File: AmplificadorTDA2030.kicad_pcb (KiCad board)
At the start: 2 copper layers, 76 x 60 mm, 45 parts, among them J1 R_Speaker, J2 SJ1-3523N, J3 DC-005, J4 L_Speaker, U1 TDA2030, U2 TDA2030

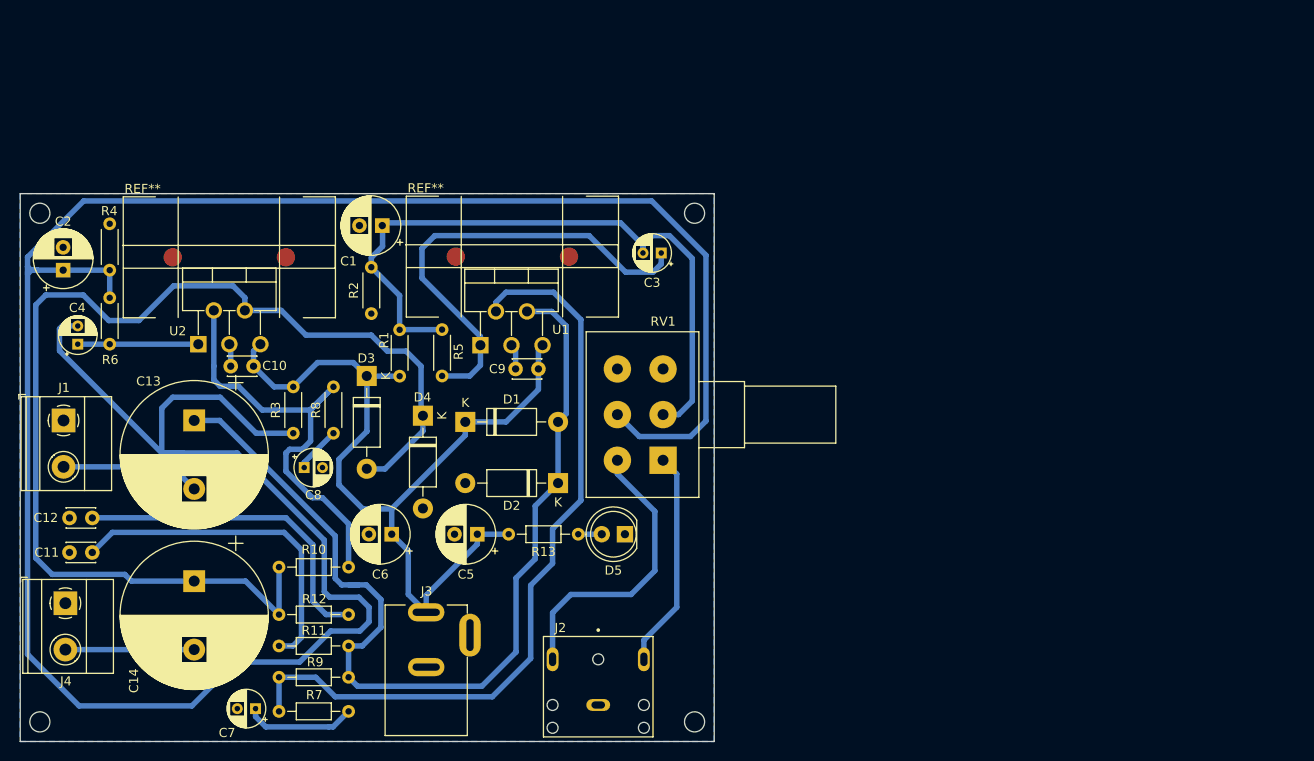
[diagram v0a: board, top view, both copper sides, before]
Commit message: Ruteo
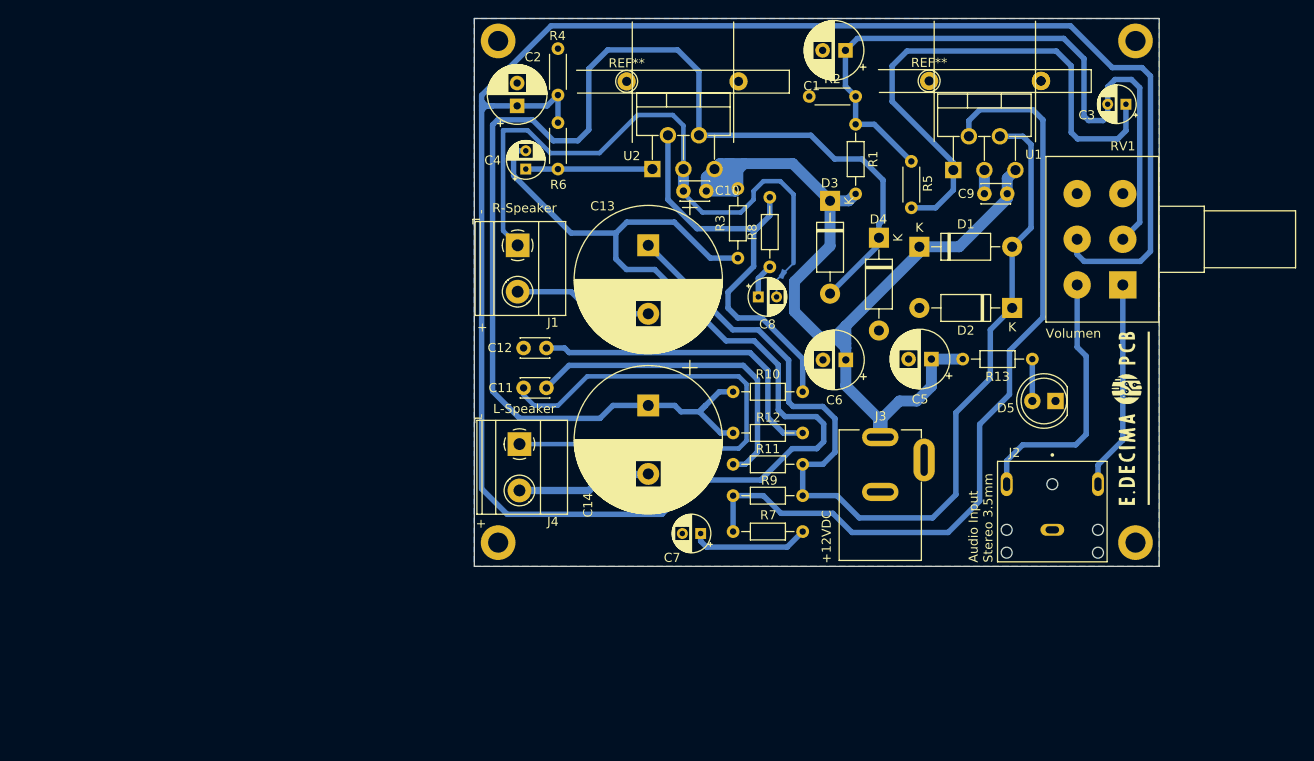
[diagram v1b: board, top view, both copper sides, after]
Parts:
- removed the ? at (136.6, 84.8)
- removed the ? at (64.8, 84.8)
- removed the ? at (64.8, 140.4)
- removed the ? at (136.6, 140.4)
- removed the REF** at (116.6, 89.5)
- removed the REF** at (85.6, 89.6)
- added ? (x2): , , F.Cu at (174.5, 70.3)
- added ?: , , F.Cu at (115.0, 120.8)
- added ?: , , F.Cu at (141.4, 70.3)
- added G***: LOGO, Logo_Image:Logo1_Decima 30mm, F.Cu at (184.2, 107.2)
- added REF**: TestPoint_THTPad_D2.0mm_Drill1.0mm, TestPoint:TestPoint_THTPad_D2.0mm_Drill1.0mm, F.Cu at (129.1, 70.3)
- added REF**: TestPoint_THTPad_D2.0mm_Drill1.0mm, TestPoint:TestPoint_THTPad_D2.0mm_Drill1.0mm, F.Cu at (162.2, 70.3)
- added REF**: MountingHole_2.2mm_M2_DIN965_Pad, MountingHole:MountingHole_2.2mm_M2_DIN965_Pad, F.Cu at (184.8, 120.8)
- added REF**: MountingHole_2.2mm_M2_DIN965_Pad, MountingHole:MountingHole_2.2mm_M2_DIN965_Pad, F.Cu at (115.0, 65.9)
- added REF**: MountingHole_2.2mm_M2_DIN965_Pad, MountingHole:MountingHole_2.2mm_M2_DIN965_Pad, F.Cu at (184.8, 65.9)
- R1, R3, R8: footprint Resistor_THT:R_Axial_DIN0204_L3.6mm_D1.6mm_P5.08mm_Horizontal -> Resistor_THT:R_Axial_DIN0204_L3.6mm_D1.6mm_P7.62mm_Horizontal
- moved U1 55.2 mm to (164.9, 80.0)
- moved C9 54.8 mm to (168.3, 82.6)
- moved R1 54.8 mm to (154.2, 75.0)
- moved R5 54.6 mm to (160.3, 79.1)
- moved D3 54.2 mm to (151.4, 83.4)
- moved C1 54.2 mm to (153.1, 66.9)
- moved RV1 53.9 mm to (183.4, 92.6)
- moved D4 53.6 mm to (156.7, 87.4)
- moved R11 53.6 mm to (140.8, 112.2)
- moved R12 53.6 mm to (148.4, 108.8)
- moved R9 53.6 mm to (148.4, 115.7)
- moved R2 53.5 mm to (149.1, 72.0), turned to 0 degrees
- moved R7 53.5 mm to (148.4, 119.6)
- moved C3 53.4 mm to (183.8, 72.8)
- moved C14 53.3 mm to (131.5, 105.8)
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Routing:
- net GND: track 5.46 -> 132.7 mm
- net Net-(D3-A): track 126.8 -> 142.6 mm
- net /V+: track 96.6 -> 107.2 mm
- net /L_Input: track 288.1 -> 277.8 mm
- net Net-(U1-+): track 50.1 -> 59.6 mm
- net Net-(U1--): track 85.3 -> 89.2 mm
- net /R_Input: track 75.1 -> 78.0 mm
- net Net-(J2-Pad3): track 32.0 -> 29.2 mm
- net Net-(U2--): track 49.3 -> 47.2 mm
- net Net-(D5-A): track 2.58 -> 4.59 mm
- net Net-(C8-Pad1): track 5.09 -> 3.81 mm
- net Net-(C12-Pad2): track 36.1 -> 34.9 mm
- net Net-(C11-Pad2): track 37.0 -> 35.9 mm
- net Net-(J2-Pad2): track 23.9 -> 22.9 mm
- net Net-(C7-Pad1): track 12.2 -> 13.0 mm
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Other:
- board size 76 x 60 mm -> 75 x 60 mm
- board text added: "+"
- board text added: "+12VDC"
- board text added: "-"
- board text added: "Audio Input Stereo 3.5mm"
- board text added: "L-Speaker"
- board text added: "R-Speaker"
- board text added: "Volumen"
